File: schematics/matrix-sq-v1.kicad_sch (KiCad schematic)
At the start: 135 parts, among them J1 trg in 2, J2 trg in 1, J3 CV1, J4 CV2, J5 CV3, J6 Power, Q1 Q_NPN_BCE, Q2 Q_NPN_BCE, SW1 SW_Push, SW2 SW_Push, SW3 SW_Push, SW4 SW_Push, U1 TL084, X1 SW_Push, X2 SW_Push, X3 SW_Push, X4 SW_Push, X5 SW_Push, X6 SW_Push, Y1 SW_Push, Y2 SW_Push, Y3 SW_Push, Y4 SW_Push, Y5 SW_Push, Y6 SW_Push, Y7 Crystal

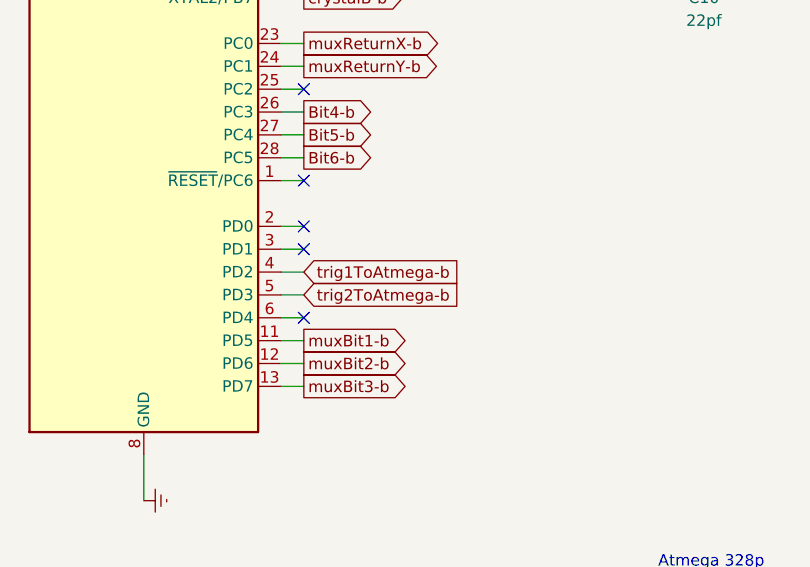
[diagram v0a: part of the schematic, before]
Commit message: pcb front and fill
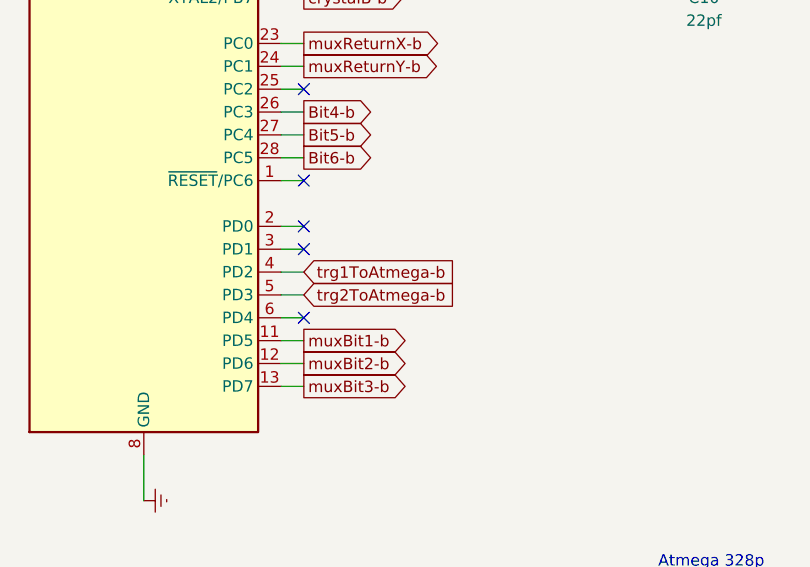
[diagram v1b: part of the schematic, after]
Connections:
- net trig1ToAtmega-b is gone; now on net trg1ToAtmega-b: Atmega1.4 (PD2)
- net trig2ToAtmega-b is gone; now on net trg2ToAtmega-b: Atmega1.5 (PD3)
